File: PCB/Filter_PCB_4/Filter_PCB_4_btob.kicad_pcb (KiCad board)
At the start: 4 copper layers, 36.6 x 8.9 mm, 45 parts, among them J1 Conn_Coaxial, J2 Conn_Coaxial, J3 Conn_01x06_Male, U1 MCP4728

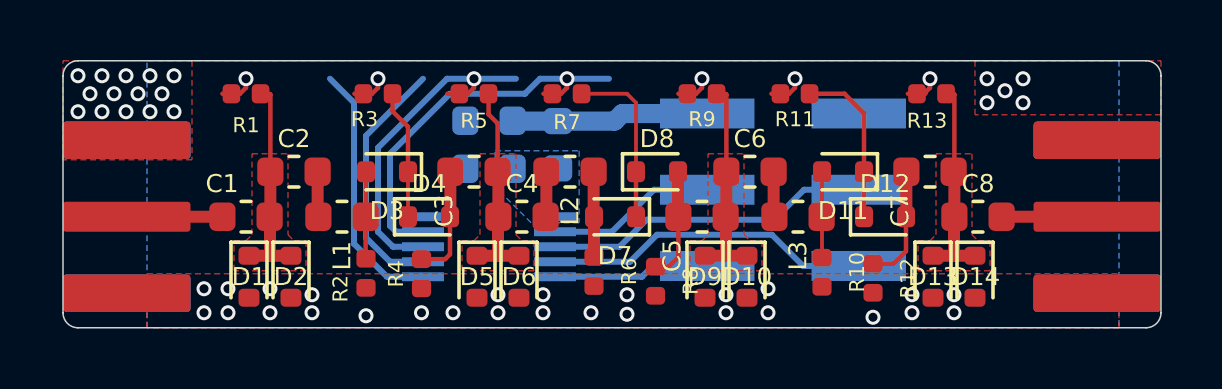
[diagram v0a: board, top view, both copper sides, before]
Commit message: pcb4 board update
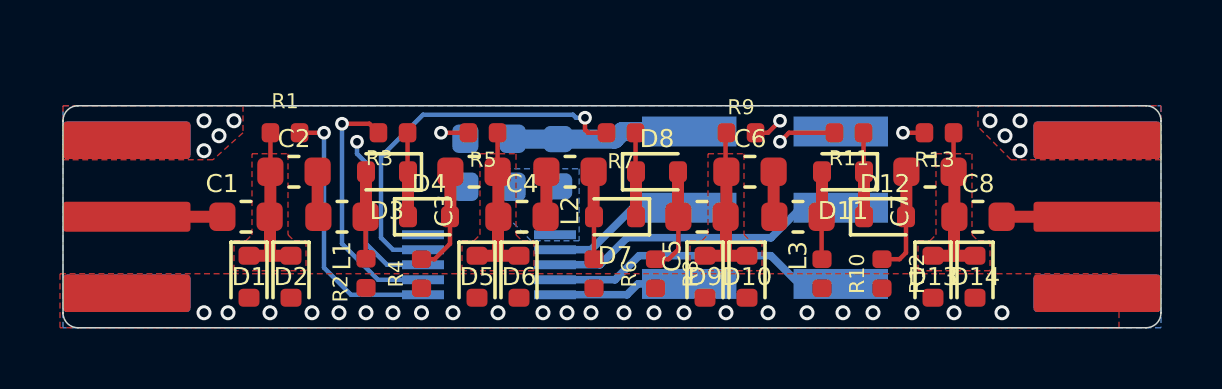
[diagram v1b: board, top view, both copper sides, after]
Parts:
- moved R11 2.22 mm to (171.9, 98.5)
- moved R7 2.22 mm to (164.3, 98.5)
- moved R9 1.84 mm to (168.3, 98.5), turned to 180 degrees
- moved R1 1.84 mm to (153.1, 98.5), turned to 180 degrees
- moved R3 1.39 mm to (156.7, 98.5)
- moved R5 1.33 mm to (159.7, 98.5)
- moved R13 1.32 mm to (174.9, 98.5)
- moved J3 0.85 mm to (169.1, 101.0)
- moved C9 0.60 mm to (159.9, 98.7)
- moved U1 0.60 mm to (159.9, 102.9)
- moved C10 0.60 mm to (159.9, 100.3)
- moved L4 0.60 mm to (162.2, 99.5)
- moved R12 0.34 mm to (173.0, 103.2)
- moved R8 0.25 mm to (165.4, 103.2)
- moved R6 0.08 mm to (163.4, 103.2)
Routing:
- net /RF/res1/Vd+: track 5.74 -> 2.81 mm
- net /RF/V1: track 23.8 -> 26.7 mm
- net /RF/V2: track 19.1 -> 22.0 mm, vias 2 -> 3
- net /RF/res2/Vd+: track 5.53 -> 2.81 mm
- net VDD: track 6.60 -> 8.33 mm
- net /RF/res0/Vd+: track 4.31 -> 2.81 mm
- net /RF/inv1/Vd: track 6.94 -> 5.52 mm
- net /RF/inv3/Vd: track 6.83 -> 5.52 mm
- net /RF/inv0/Vd: track 6.83 -> 5.52 mm
- net /RF/inv2/Vd: track 6.83 -> 5.53 mm
- net /RF/V0: track 30.6 -> 31.8 mm
- net /DAC/~LDAC: track 11.8 -> 10.8 mm
- net /DAC/SDA: track 11.8 -> 10.9 mm
- net /DAC/RDY: track 6.12 -> 5.22 mm
- net /DAC/SCL: track 6.55 -> 5.65 mm
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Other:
- board size 36.6 x 8.9 mm -> 36.6 x 7.4 mm
